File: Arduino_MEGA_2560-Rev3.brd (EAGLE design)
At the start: 111.3 x 99 mm, 49 parts

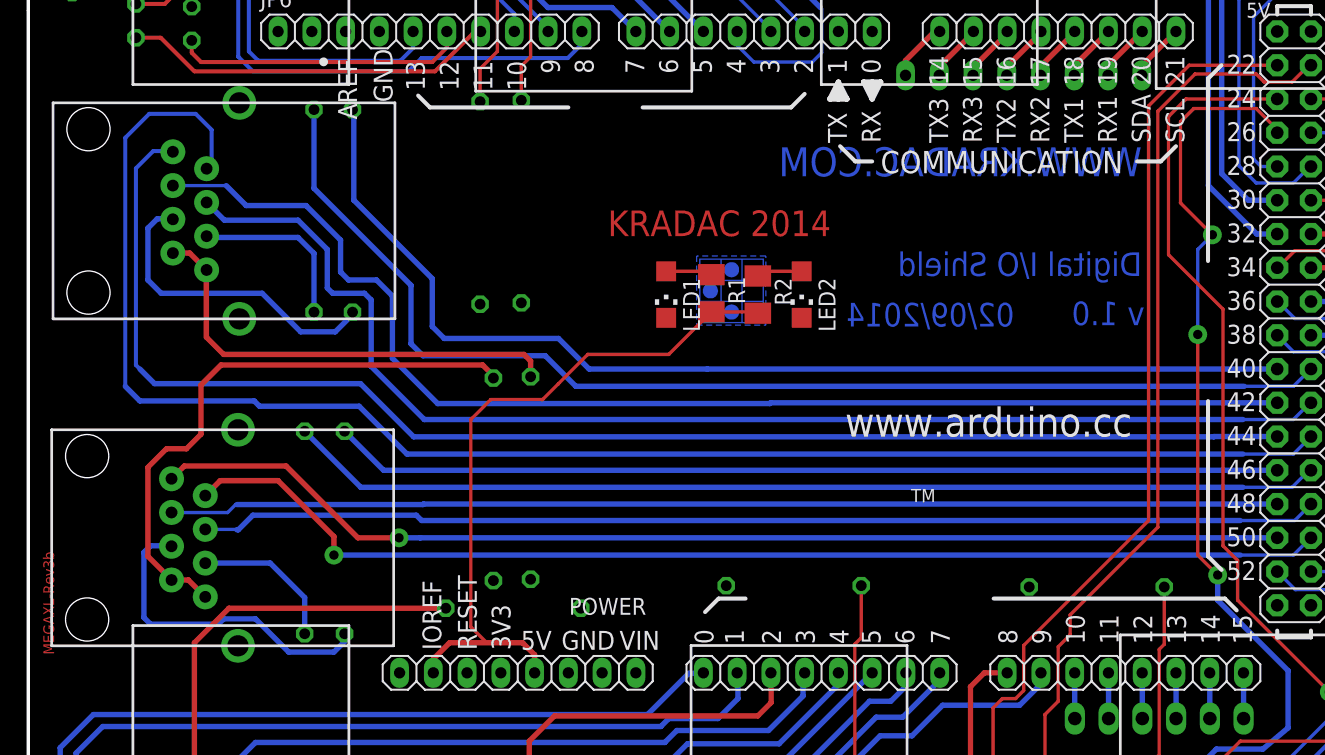
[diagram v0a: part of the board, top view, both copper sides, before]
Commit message: Terminada la version 1.0
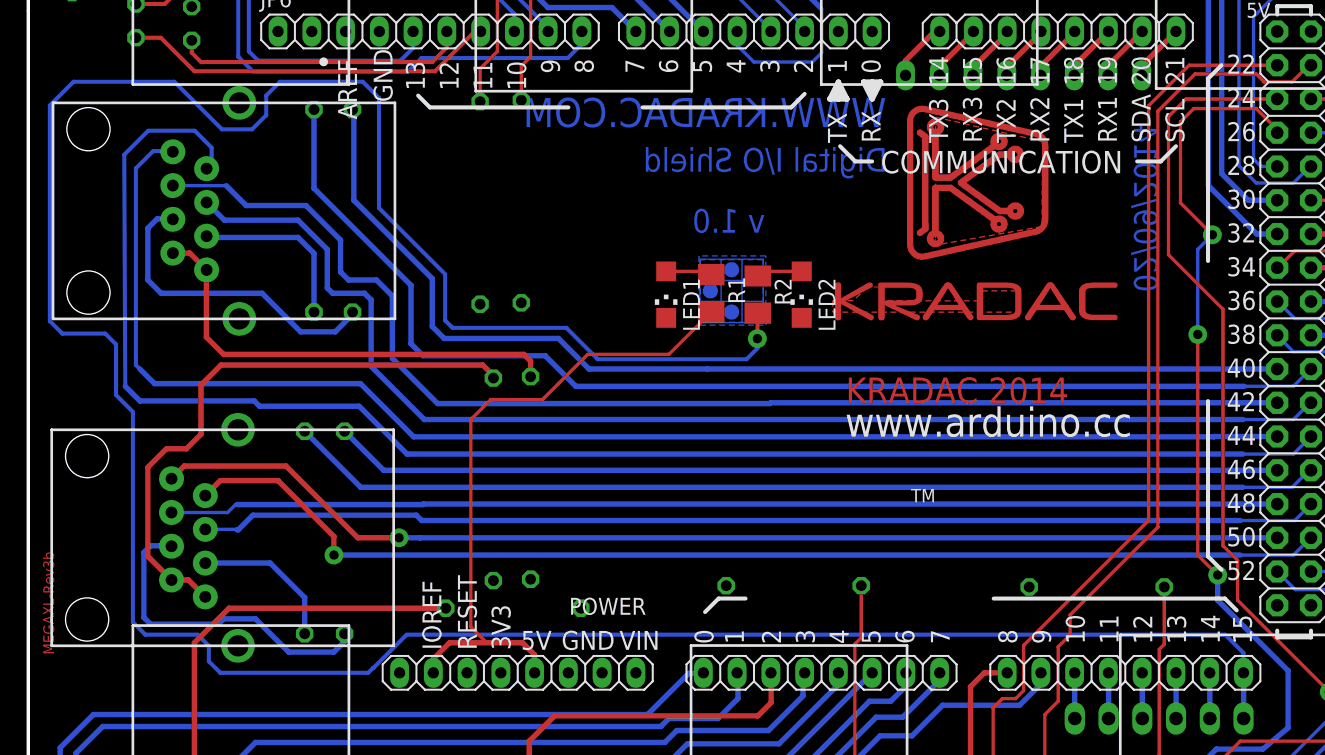
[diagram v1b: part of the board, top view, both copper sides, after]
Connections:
- net GND renamed COUT_GND
- net +5V: no longer R2.2
- net N$25: now also R2.2
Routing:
- net N$25: track 3.45 -> 212.2 mm, vias 0 -> 1
- net +5V: track 55.9 -> 52.4 mm
- net PL4: track 121.4 -> 118.9 mm
- added copper zone on layer 1, net N$47
- added copper zone on layer 1, net N$48
- added copper zone on layer 16, net N$49
- added copper zone on layer 16, net N$50
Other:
- board text added: "C:/Users/Ernesto/eagle/KRADAC/Logo_Kradac_Eagle.bmp"
